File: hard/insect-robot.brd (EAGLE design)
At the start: 10.2 x 25.4 mm, 12 parts, among them SW1 SWITCH-DT, U1 ATMEGA328P-QFN32, U2 PW0316

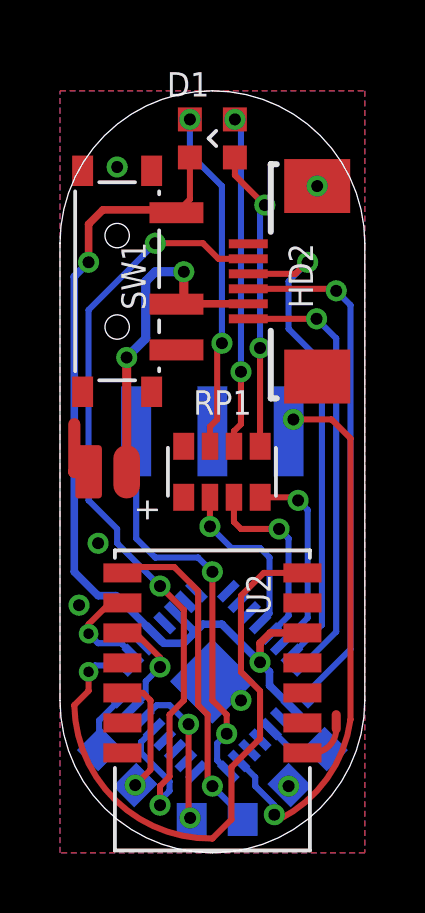
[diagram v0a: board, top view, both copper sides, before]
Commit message: PWM pins
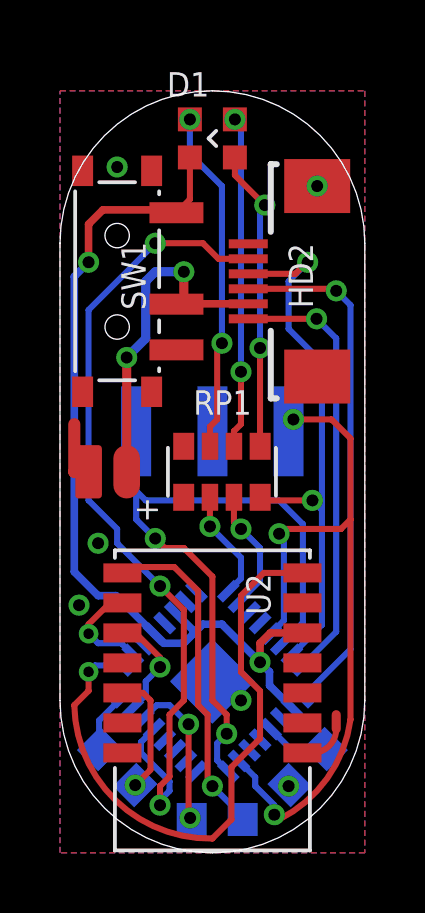
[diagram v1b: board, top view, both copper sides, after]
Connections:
- removed net MOSI: HD2.4, U1.15
- removed net RB-: RP1.8, U1.14
- new net RB-/MOSI: HD2.4, RP1.8, U1.15
- net L: now also U1.14
- net R: now also U1.13
- net RG-: now also U1.10; no longer U1.13
- net RR-: now also U1.9; no longer U1.12
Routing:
- net RB-/MOSI: track 0.00 -> 18.6 mm, vias 0 -> 2
- net MOSI: track 16.4 -> 0.00 mm, vias 1 -> 0
- net L: track 13.7 -> 23.6 mm
- net RB-: track 6.60 -> 0.00 mm, vias 1 -> 0
- net R: track 18.6 -> 24.8 mm, vias 2 -> 3
- net RG-: track 6.29 -> 4.14 mm
- net RR-: track 5.70 -> 3.73 mm
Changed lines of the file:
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@@
 <contactref element="HD1" pad="1"/>
 <contactref element="U1" pad="24"/>
-<wire x1="2.54" y1="10.4775" x2="2.54" y2="14.05" width="0.2032" layer="16"/>
-<wire x1="2.54" y1="10.4775" x2="3.175" y2="9.8425" width="0.2032" layer="16"/>
+<wire x1="2.54" y1="12.065" x2="2.54" y2="14.05" width="0.2032" layer="16"/>
 <via x="5.55625" y="3.96875" extent="1-16" drill="0.4"/>
 <wire x1="5.55625" y1="4.60375" x2="5.08" y2="5.08" width="0.2032" layer="1"/>
-<wire x1="5.08" y1="5.08" x2="5.08" y2="9.36625" width="0.2032" layer="1"/>
-<via x="5.08" y="9.36625" extent="1-16" drill="0.4"/>
-<wire x1="5.08" y1="9.36625" x2="4.60375" y2="9.8425" width="0.2032" layer="16"/>
-<wire x1="4.60375" y1="9.8425" x2="3.175" y2="9.8425" width="0.2032" layer="16"/>
 <wire x1="5.55625" y1="4.60375" x2="5.55625" y2="3.96875" width="0.2032" layer="1"/>
 <wire x1="5.55625" y1="3.96875" x2="5.23875" y2="3.65125" width="0.2032" layer="16"/>
 <wire x1="5.23875" y1="3.65125" x2="5.23875" y2="3.081375" width="0.2032" layer="16"/>
 <wire x1="5.23875" y1="3.081375" x2="5.61033125" y2="2.70979375" width="0.2032" layer="16"/>
+<contactref element="U1" pad="14"/>
+<wire x1="7.3781" y1="6.952434375" x2="8.09625" y2="7.670584375" width="0.2032" layer="16"/>
+<wire x1="7.3025" y1="11.7475" x2="2.8575" y2="11.7475" width="0.2032" layer="16"/>
+<wire x1="2.8575" y1="11.7475" x2="2.54" y2="12.065" width="0.2032" layer="16"/>
+<wire x1="5.08" y1="5.08" x2="5.08" y2="9.2075" width="0.2032" layer="1"/>
+<wire x1="5.08" y1="9.2075" x2="4.1275" y2="10.16" width="0.2032" layer="1"/>
+<wire x1="4.1275" y1="10.16" x2="3.4925" y2="10.16" width="0.2032" layer="1"/>
+<wire x1="3.4925" y1="10.16" x2="3.175" y2="10.4775" width="0.2032" layer="1"/>
+<via x="3.175" y="10.4775" extent="1-16" drill="0.4"/>
+<wire x1="3.175" y1="10.4775" x2="2.54" y2="11.1125" width="0.2032" layer="16"/>
+<wire x1="2.54" y1="11.1125" x2="2.54" y2="12.065" width="0.2032" layer="16"/>
+<wire x1="8.09625" y1="7.670584375" x2="8.09625" y2="10.95375" width="0.2032" layer="16"/>
+<wire x1="8.09625" y1="10.95375" x2="7.3025" y2="11.7475" width="0.2032" layer="16"/>
 </signal>
 <signal name="R">
@@
 <wire x1="6.50875" y1="2.51848125" x2="5.963884375" y2="3.063346875" width="0.2032" layer="16"/>
 <via x="7.77875" y="14.44625" extent="1-16" drill="0.4"/>
-<wire x1="9.68375" y1="4.445" x2="9.68375" y2="13.81125" width="0.2032" layer="1"/>
+<wire x1="9.68375" y1="4.445" x2="9.68375" y2="11.1125" width="0.2032" layer="1"/>
+<wire x1="9.68375" y1="11.1125" x2="9.68375" y2="13.81125" width="0.2032" layer="1"/>
 <wire x1="9.68375" y1="13.81125" x2="9.04875" y2="14.44625" width="0.2032" layer="1"/>
 <wire x1="9.04875" y1="14.44625" x2="7.77875" y2="14.44625" width="0.2032" layer="1"/>
 <wire x1="7.77875" y1="14.44625" x2="7.62" y2="14.2875" width="0.2032" layer="16"/>
 <wire x1="7.62" y1="14.2875" x2="7.62" y2="14.05" width="0.2032" layer="16"/>
+<contactref element="U1" pad="13"/>
+<wire x1="7.02454375" y1="7.3059875" x2="7.46125" y2="7.74269375" width="0.2032" layer="16"/>
+<wire x1="7.46125" y1="10.4775" x2="7.3025" y2="10.63625" width="0.2032" layer="16"/>
+<via x="7.3025" y="10.63625" extent="1-16" drill="0.4"/>
+<wire x1="7.3025" y1="10.63625" x2="7.46125" y2="10.795" width="0.2032" layer="1"/>
+<wire x1="7.46125" y1="10.795" x2="9.36625" y2="10.795" width="0.2032" layer="1"/>
+<wire x1="9.36625" y1="10.795" x2="9.68375" y2="11.1125" width="0.2032" layer="1"/>
+<wire x1="7.46125" y1="7.74269375" x2="7.46125" y2="10.4775" width="0.2032" layer="16"/>
 </signal>
 <signal name="RXD">
@@
 <wire x1="5.715" y1="1.11125" x2="5.08" y2="0.47625" width="0.2032" layer="1"/>
 </signal>
-<signal name="MOSI">
+<signal name="RB-/MOSI">
 <contactref element="U1" pad="15"/>
 <contactref element="HD2" pad="4"/>
@@
 <wire x1="7.62" y1="17.4625" x2="7.62" y2="19.05" width="0.2032" layer="16"/>
 <wire x1="7.62" y1="19.05" x2="8.255" y2="19.685" width="0.2032" layer="16"/>
-<wire x1="8.73125" y1="7.598478125" x2="8.73125" y2="16.35125" width="0.2032" layer="16"/>
 <wire x1="8.73125" y1="16.35125" x2="7.62" y2="17.4625" width="0.2032" layer="16"/>
+<contactref element="RP1" pad="8"/>
+<wire x1="6.6725" y1="11.85" x2="6.775" y2="11.7475" width="0.2032" layer="1"/>
+<wire x1="6.775" y1="11.7475" x2="8.41375" y2="11.7475" width="0.2032" layer="1"/>
+<via x="8.41375" y="11.7475" extent="1-16" drill="0.4"/>
+<wire x1="8.73125" y1="7.598478125" x2="8.73125" y2="11.43" width="0.2032" layer="16"/>
+<wire x1="8.73125" y1="11.43" x2="8.73125" y2="16.35125" width="0.2032" layer="16"/>
+<wire x1="8.41375" y1="11.7475" x2="8.73125" y2="11.43" width="0.2032" layer="16"/>
 </signal>
 <signal name="MISO">
@@
 <wire x1="6.275" y1="18.3" x2="3.895" y2="18.3" width="0.254" layer="1"/>
 <wire x1="3.895" y1="18.3" x2="3.883" y2="18.288" width="0.254" layer="1"/>
-</signal>
-<signal name="RR-">
-<contactref element="U1" pad="12"/>
-<contactref element="RP1" pad="4"/>
-<wire x1="6.670990625" y1="7.659540625" x2="6.985" y2="7.97355" width="0.2032" layer="16"/>
-<wire x1="6.985" y1="7.97355" x2="6.985" y2="9.8425" width="0.2032" layer="16"/>
-<wire x1="6.985" y1="9.8425" x2="6.6675" y2="10.16" width="0.2032" layer="16"/>
-<wire x1="6.6675" y1="10.16" x2="5.715" y2="10.16" width="0.2032" layer="16"/>
-<wire x1="5.715" y1="10.16" x2="4.9975" y2="10.8775" width="0.2032" layer="16"/>
-<via x="4.9975" y="10.8775" extent="1-16" drill="0.4"/>
-<wire x1="4.9975" y1="10.8775" x2="4.9975" y2="11.85" width="0.2032" layer="1"/>
-</signal>
-<signal name="RG-">
-<contactref element="U1" pad="13"/>
-<contactref element="RP1" pad="6"/>
-<wire x1="7.02454375" y1="7.3059875" x2="7.62" y2="7.90144375" width="0.2032" layer="16"/>
-<wire x1="7.62" y1="7.90144375" x2="7.62" y2="10.4775" width="0.2032" layer="16"/>
-<wire x1="7.62" y1="10.4775" x2="7.3025" y2="10.795" width="0.2032" layer="16"/>
-<via x="7.3025" y="10.795" extent="1-16" drill="0.4"/>
-<wire x1="7.3025" y1="10.795" x2="6.0325" y2="10.795" width="0.2032" layer="1"/>
-<wire x1="6.0325" y1="10.795" x2="5.7975" y2="11.03" width="0.2032" layer="1"/>
-<wire x1="5.7975" y1="11.03" x2="5.7975" y2="11.85" width="0.2032" layer="1"/>
-</signal>
-<signal name="RB-">
-<contactref element="U1" pad="14"/>
-<contactref element="RP1" pad="8"/>
-<wire x1="7.3781" y1="6.952434375" x2="8.255" y2="7.829334375" width="0.2032" layer="16"/>
-<wire x1="8.255" y1="7.829334375" x2="8.255" y2="11.43" width="0.2032" layer="16"/>
-<wire x1="8.255" y1="11.43" x2="7.9375" y2="11.7475" width="0.2032" layer="16"/>
-<via x="7.9375" y="11.7475" extent="1-16" drill="0.4"/>
-<wire x1="7.9375" y1="11.7475" x2="7.835" y2="11.85" width="0.2032" layer="1"/>
-<wire x1="7.835" y1="11.85" x2="6.6725" y2="11.85" width="0.2032" layer="1"/>
 </signal>
 <signal name="R-">
@@
 <wire x1="0.9525" y1="11.7475" x2="0.9525" y2="18.0975" width="0.2032" layer="16"/>
 </signal>
+<signal name="RR-">
+<contactref element="RP1" pad="4"/>
+<contactref element="U1" pad="9"/>
+<wire x1="4.9975" y1="10.8775" x2="6.0325" y2="9.8425" width="0.2032" layer="16"/>
+<wire x1="6.0325" y1="9.8425" x2="6.0325" y2="9.142371875" width="0.2032" layer="16"/>
+<wire x1="6.0325" y1="9.142371875" x2="5.61033125" y2="8.720203125" width="0.2032" layer="16"/>
+<via x="4.9975" y="10.8775" extent="1-16" drill="0.4"/>
+<wire x1="4.9975" y1="10.8775" x2="4.9975" y2="11.85" width="0.2032" layer="1"/>
+</signal>
+<signal name="RG-">
+<contactref element="RP1" pad="6"/>
+<contactref element="U1" pad="10"/>
+<wire x1="5.963884375" y1="8.36665" x2="6.6675" y2="9.070265625" width="0.2032" layer="16"/>
+<wire x1="5.7975" y1="11.03" x2="5.7975" y2="11.85" width="0.2032" layer="1"/>
+<wire x1="6.6675" y1="9.070265625" x2="6.6675" y2="10.16" width="0.2032" layer="16"/>
+<wire x1="6.6675" y1="10.16" x2="6.0325" y2="10.795" width="0.2032" layer="16"/>
+<via x="6.0325" y="10.795" extent="1-16" drill="0.4"/>
+<wire x1="6.0325" y1="10.795" x2="5.7975" y2="11.03" width="0.2032" layer="1"/>
+</signal>
 </signals>
